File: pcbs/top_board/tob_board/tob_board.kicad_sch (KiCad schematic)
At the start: 7 parts, among them J1 LEDFrontRight, J2 LEDRearRight, J3 LEDFrontLeft, J4 LEDRearLeft, J5 Motor, J6 Motor1, J7 Motor2

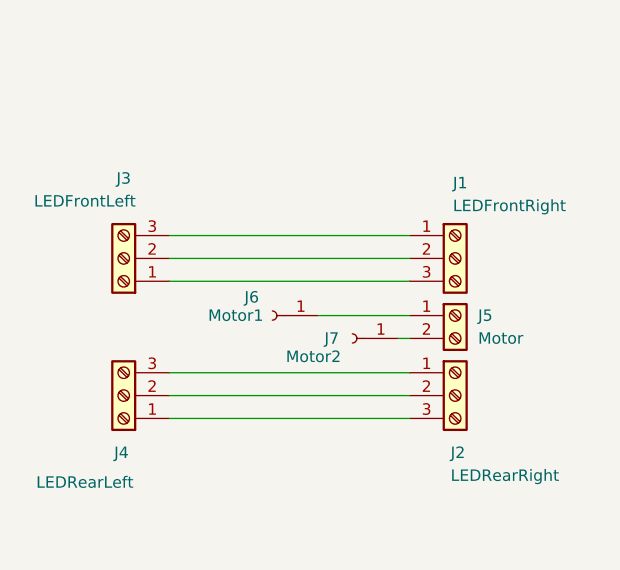
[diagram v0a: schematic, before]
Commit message: board update
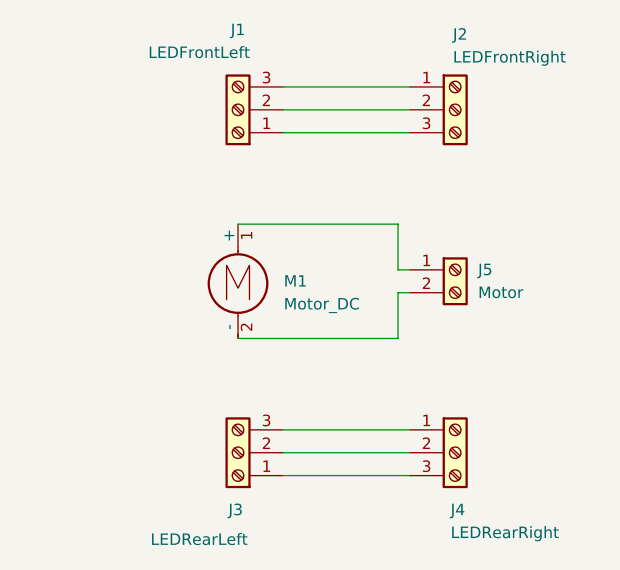
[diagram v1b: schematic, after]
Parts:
- removed J6: Motor1, Connector_Pin:Pin_D1.0mm_L10.0mm_LooseFit, symbol Connector:Conn_01x01_Socket
- removed J7: Motor2, Connector_Pin:Pin_D1.0mm_L10.0mm_LooseFit, symbol Connector:Conn_01x01_Socket
- added M1: Motor_DC, topMotor:topMotor, symbol Motor:Motor_DC
- renumbered J3 to J1, J1 to J2, J4 to J3, J2 to J4
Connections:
- net at J5.1 (Pin_1): now also M1.1 (+)
- net at J5.2 (Pin_2): now also M1.2 (-)
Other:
- moved on the sheet: J1, J2, J3, J4, J5

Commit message: ID pins, BOM, fuse
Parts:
- J1, J2, J3, J4: Manufacturer Part Number (none) -> S3B-XH-A-E(LF)(SN); Supplier (none) -> Mouser; Supplier Part Number (none) -> 306-S3BXHAELFSN
- J5: Manufacturer Part Number (none) -> S2B-XH-A-BK(LF)(SN); Supplier (none) -> Mouser; Supplier Part Number (none) -> 306-S2BXHABKLFSN
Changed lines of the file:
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@@
 			)
 		)
-		(property "Datasheet" "~"
+		(property "Datasheet" "https://cz.mouser.com/datasheet/3/1070/1/eXH.pdf"
 			(at 190.5 50.8 0)
 			(effects
@@
 			)
 		)
-		(property "Description" "Generic screw terminal, single row, 01x03, script generated (kicad-library-utils/schlib/autogen/connector/)"
+		(property "Description" "JST XH 3 pin, zásuvka, boční"
+			(at 190.5 50.8 0)
+			(effects
+				(font
+					(size 1.27 1.27)
+				)
+				(hide yes)
+			)
+		)
+		(property "Manufacturer Part Number" "S3B-XH-A-E(LF)(SN)"
+			(at 190.5 50.8 0)
+			(effects
+				(font
+					(size 1.27 1.27)
+				)
+				(hide yes)
+			)
+		)
+		(property "Supplier" "Mouser"
+			(at 190.5 50.8 0)
+			(effects
+				(font
+					(size 1.27 1.27)
+				)
+				(hide yes)
+			)
+		)
+		(property "Supplier Part Number" "306-S3BXHAELFSN"
 			(at 190.5 50.8 0)
 			(effects
@@
 			)
 		)
-		(property "Datasheet" "~"
+		(property "Datasheet" "https://cz.mouser.com/datasheet/3/1070/1/eXH.pdf"
 			(at 190.5 88.9 0)
 			(effects
@@
 			)
 		)
-		(property "Description" "Generic screw terminal, single row, 01x03, script generated (kicad-library-utils/schlib/autogen/connector/)"
+		(property "Description" "JST XH 3 pin, zásuvka, boční"
+			(at 190.5 88.9 0)
+			(effects
+				(font
+					(size 1.27 1.27)
+				)
+				(hide yes)
+			)
+		)
+		(property "Manufacturer Part Number" "S3B-XH-A-E(LF)(SN)"
+			(at 190.5 88.9 0)
+			(effects
+				(font
+					(size 1.27 1.27)
+				)
+				(hide yes)
+			)
+		)
+		(property "Supplier" "Mouser"
+			(at 190.5 88.9 0)
+			(effects
+				(font
+					(size 1.27 1.27)
+				)
+				(hide yes)
+			)
+		)
+		(property "Supplier Part Number" "306-S3BXHAELFSN"
 			(at 190.5 88.9 0)
 			(effects
@@
 			)
 		)
+		(property "Manufacturer Part Number" ""
+			(at 166.37 68.58 0)
+			(effects
+				(font
+					(size 1.27 1.27)
+				)
+				(hide yes)
+			)
+		)
+		(property "Supplier" ""
+			(at 166.37 68.58 0)
+			(effects
+				(font
+					(size 1.27 1.27)
+				)
+				(hide yes)
+			)
+		)
+		(property "Supplier Part Number" ""
+			(at 166.37 68.58 0)
+			(effects
+				(font
+					(size 1.27 1.27)
+				)
+				(hide yes)
+			)
+		)
 		(pin "2"
 		)
@@
 			)
 		)
-		(property "Datasheet" "~"
+		(property "Datasheet" "https://cz.mouser.com/datasheet/3/1070/1/eXH.pdf"
 			(at 166.37 88.9 0)
 			(effects
@@
 			)
 		)
-		(property "Description" "Generic screw terminal, single row, 01x03, script generated (kicad-library-utils/schlib/autogen/connector/)"
+		(property "Description" "JST XH 3 pin, zásuvka, boční"
+			(at 166.37 88.9 0)
+			(effects
+				(font
+					(size 1.27 1.27)
+				)
+				(hide yes)
+			)
+		)
+		(property "Manufacturer Part Number" "S3B-XH-A-E(LF)(SN)"
+			(at 166.37 88.9 0)
+			(effects
+				(font
+					(size 1.27 1.27)
+				)
+				(hide yes)
+			)
+		)
+		(property "Supplier" "Mouser"
+			(at 166.37 88.9 0)
+			(effects
+				(font
+					(size 1.27 1.27)
+				)
+				(hide yes)
+			)
+		)
+		(property "Supplier Part Number" "306-S3BXHAELFSN"
 			(at 166.37 88.9 0)
 			(effects
@@
 			)
 		)
-		(property "Datasheet" "~"
+		(property "Datasheet" "https://cz.mouser.com/datasheet/3/1070/1/eXH.pdf"
 			(at 166.37 50.8 0)
 			(effects
@@
 			)
 		)
-		(property "Description" "Generic screw terminal, single row, 01x03, script generated (kicad-library-utils/schlib/autogen/connector/)"
+		(property "Description" "JST XH 3 pin, zásuvka, boční"
+			(at 166.37 50.8 0)
+			(effects
+				(font
+					(size 1.27 1.27)
+				)
+				(hide yes)
+			)
+		)
+		(property "Manufacturer Part Number" "S3B-XH-A-E(LF)(SN)"
+			(at 166.37 50.8 0)
+			(effects
+				(font
+					(size 1.27 1.27)
+				)
+				(hide yes)
+			)
+		)
+		(property "Supplier" "Mouser"
+			(at 166.37 50.8 0)
+			(effects
+				(font
+					(size 1.27 1.27)
+				)
+				(hide yes)
+			)
+		)
+		(property "Supplier Part Number" "306-S3BXHAELFSN"
 			(at 166.37 50.8 0)
 			(effects
@@
 			)
 		)
-		(property "Datasheet" "~"
+		(property "Datasheet" "https://cz.mouser.com/datasheet/3/1070/1/eXH.pdf"
 			(at 190.5 68.58 0)
 			(effects
@@
 			)
 		)
-		(property "Description" "Generic screw terminal, single row, 01x02, script generated (kicad-library-utils/schlib/autogen/connector/)"
+		(property "Description" "JST XH 2 pin, zásuvka, boční"
 			(at 190.5 68.58 0)
 			(effects
+				(font
+					(size 1.27 1.27)
+				)
+				(hide yes)
+			)
+		)
+		(property "Manufacturer Part Number" "S2B-XH-A-BK(LF)(SN)"
+			(at 190.5 68.58 0)
+			(effects
+				(font
+					(size 1.27 1.27)
+				)
+				(hide yes)
+			)
+		)
+		(property "Supplier" "Mouser"
+			(at 190.5 68.58 0)
+			(effects
+				(font
+					(size 1.27 1.27)
+				)
+				(hide yes)
+			)
+		)
+		(property "Supplier Part Number" "306-S2BXHABKLFSN"
+			(at 190.5 68.58 0)
+			(effects

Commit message: Add edge cuts and notes to pcb
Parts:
- M1: Manufacturer Part Number (none) -> LA143024A; Supplier (none) -> LaskaKit; Supplier Part Number (none) -> LA143024A
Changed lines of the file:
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@@
 			)
 		)
-		(property "Manufacturer Part Number" ""
+		(property "Manufacturer Part Number" "LA143024A"
 			(at 166.37 68.58 0)
 			(effects
@@
 			)
 		)
-		(property "Supplier" ""
+		(property "Supplier" "LaskaKit"
 			(at 166.37 68.58 0)
 			(effects
@@
 			)
 		)
-		(property "Supplier Part Number" ""
+		(property "Supplier Part Number" "LA143024A"
 			(at 166.37 68.58 0)
 			(effects

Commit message: Components update
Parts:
- J1, J2, J3, J4: Manufacturer Part Number S3B-XH-A-E(LF)(SN) -> S3B-XH-A-1 (LF)(SN); Supplier Mouser -> TME; Supplier Part Number 306-S3BXHAELFSN -> S3B-XH-A-1
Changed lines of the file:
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@@
 			)
 		)
-		(property "Manufacturer Part Number" "S3B-XH-A-E(LF)(SN)"
+		(property "Manufacturer Part Number" "S3B-XH-A-1 (LF)(SN)"
 			(at 190.5 50.8 0)
 			(effects
@@
 			)
 		)
-		(property "Supplier" "Mouser"
+		(property "Supplier" "TME"
 			(at 190.5 50.8 0)
 			(effects
@@
 			)
 		)
-		(property "Supplier Part Number" "306-S3BXHAELFSN"
+		(property "Supplier Part Number" "S3B-XH-A-1"
 			(at 190.5 50.8 0)
 			(effects
@@
 			)
 		)
-		(property "Manufacturer Part Number" "S3B-XH-A-E(LF)(SN)"
-			(at 190.5 88.9 0)
-			(effects
-				(font
-					(size 1.27 1.27)
-				)
-				(hide yes)
-			)
-		)
-		(property "Supplier" "Mouser"
-			(at 190.5 88.9 0)
-			(effects
-				(font
-					(size 1.27 1.27)
-				)
-				(hide yes)
-			)
-		)
-		(property "Supplier Part Number" "306-S3BXHAELFSN"
+		(property "Manufacturer Part Number" "S3B-XH-A-1 (LF)(SN)"
+			(at 190.5 88.9 0)
+			(effects
+				(font
+					(size 1.27 1.27)
+				)
+				(hide yes)
+			)
+		)
+		(property "Supplier" "TME"
+			(at 190.5 88.9 0)
+			(effects
+				(font
+					(size 1.27 1.27)
+				)
+				(hide yes)
+			)
+		)
+		(property "Supplier Part Number" "S3B-XH-A-1"
 			(at 190.5 88.9 0)
 			(effects
@@
 			)
 		)
-		(property "Manufacturer Part Number" "S3B-XH-A-E(LF)(SN)"
-			(at 166.37 88.9 0)
-			(effects
-				(font
-					(size 1.27 1.27)
-				)
-				(hide yes)
-			)
-		)
-		(property "Supplier" "Mouser"
-			(at 166.37 88.9 0)
-			(effects
-				(font
-					(size 1.27 1.27)
-				)
-				(hide yes)
-			)
-		)
-		(property "Supplier Part Number" "306-S3BXHAELFSN"
+		(property "Manufacturer Part Number" "S3B-XH-A-1 (LF)(SN)"
+			(at 166.37 88.9 0)
+			(effects
+				(font
+					(size 1.27 1.27)
+				)
+				(hide yes)
+			)
+		)
+		(property "Supplier" "TME"
+			(at 166.37 88.9 0)
+			(effects
+				(font
+					(size 1.27 1.27)
+				)
+				(hide yes)
+			)
+		)
+		(property "Supplier Part Number" "S3B-XH-A-1"
 			(at 166.37 88.9 0)
 			(effects
@@
 			)
 		)
-		(property "Manufacturer Part Number" "S3B-XH-A-E(LF)(SN)"
-			(at 166.37 50.8 0)
-			(effects
-				(font
-					(size 1.27 1.27)
-				)
-				(hide yes)
-			)
-		)
-		(property "Supplier" "Mouser"
-			(at 166.37 50.8 0)
-			(effects
-				(font
-					(size 1.27 1.27)
-				)
-				(hide yes)
-			)
-		)
-		(property "Supplier Part Number" "306-S3BXHAELFSN"
-			(at 166.37 50.8 0)
-			(effects
+		(property "Manufacturer Part Number" "S3B-XH-A-1 (LF)(SN)"
+			(at 166.37 50.8 0)
+			(effects
+				(font
+					(size 1.27 1.27)
+				)
+				(hide yes)
+			)
+		)
+		(property "Supplier" "TME"
+			(at 166.37 50.8 0)
+			(effects
+				(font
+					(size 1.27 1.27)
+				)
+				(hide yes)
+			)
+		)
+		(property "Supplier Part Number" "S3B-XH-A-1"
+			(at 166.37 50.8 0)
+			(effects
